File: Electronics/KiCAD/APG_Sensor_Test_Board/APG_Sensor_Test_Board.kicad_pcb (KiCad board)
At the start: 4 copper layers, 100 x 40.6 mm, 96 parts, among them J1 Conn_01x02, J2 Conn_01x06, J3 Conn_01x02, J4 USB_C_Receptacle_USB2.0_16P, Q1 RE1C002UNTCL, SW1 SW_SPST, SW2 SW_SPST, SW3 SW_SPST, SW4 SW_SPST, U1 ESP32-S3-WROOM-1, U2 BNO085, U3 ADXL375, U4 MS5607-02BA, U5 W25Q128JVS, U6 USBULC6-2M6, U7 TLV75533PDBV

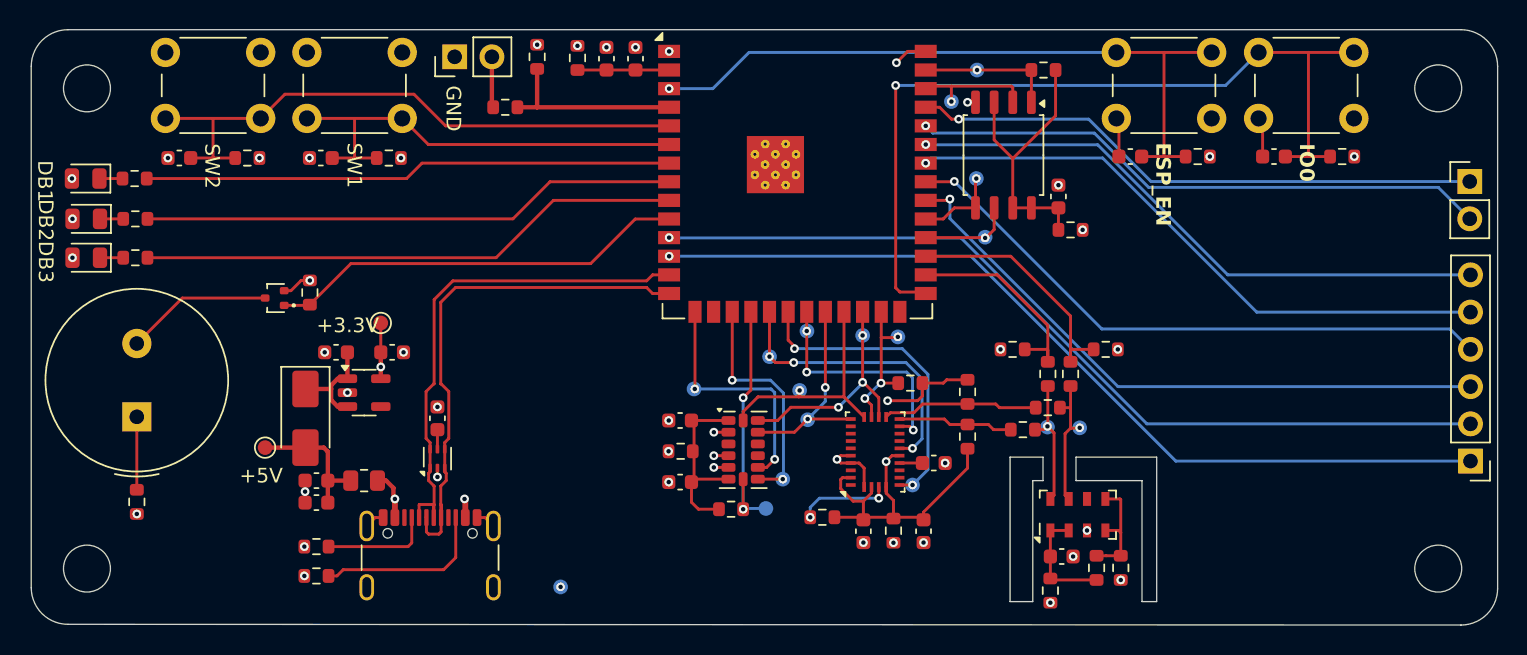
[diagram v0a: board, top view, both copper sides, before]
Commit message: APG Sensor Board V1.1 Production
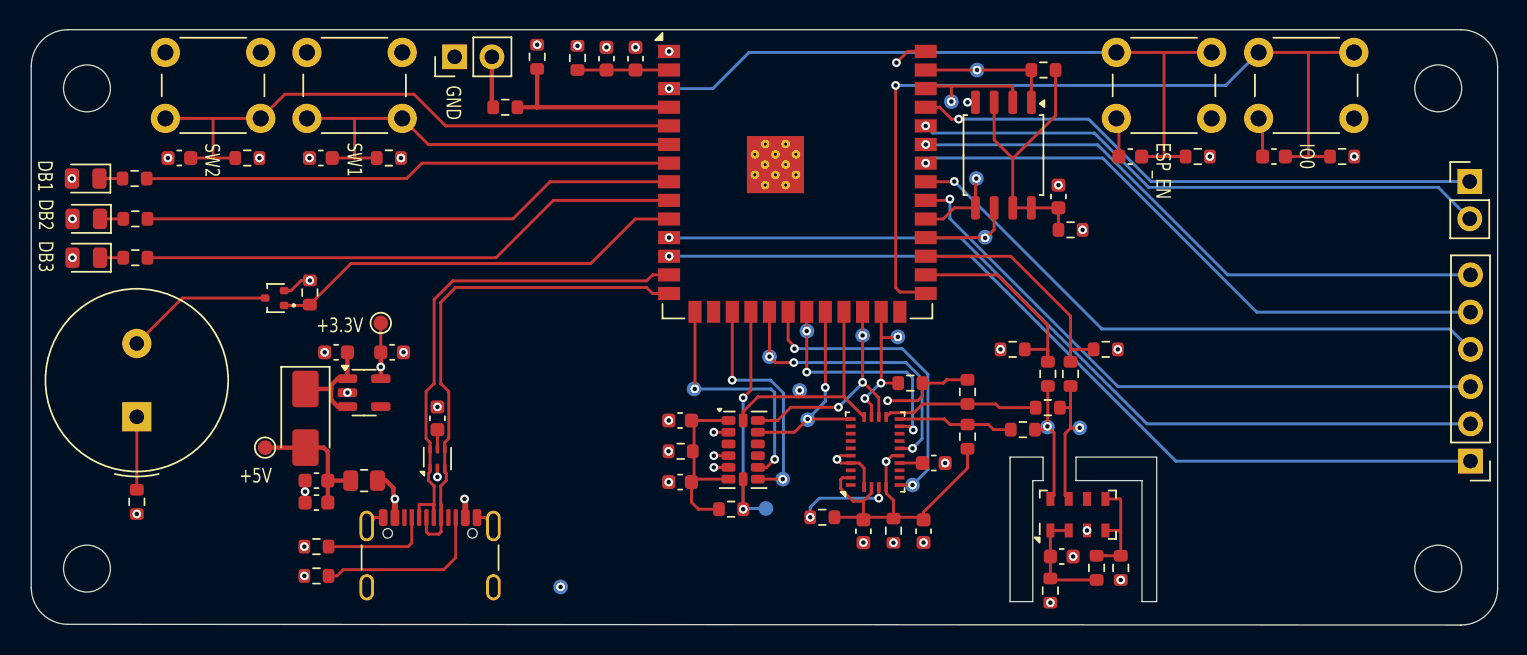
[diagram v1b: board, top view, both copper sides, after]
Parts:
- moved G*** 4.73 mm to (180.2, 68.2)
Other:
- board text added: "APG_Sensor_Board_V1.1 Gannon Bird Ethan Benne Nathan Emerson Tannyr Singleterry"
